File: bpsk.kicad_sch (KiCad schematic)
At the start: 0 parts

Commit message: update bpsk sch
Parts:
- added C1, C8: 47n, symbol Device:C
- added C18: 100n, symbol Device:C
- added C2: 10n, symbol Device:C
- added J1: Screw_Terminal_01x03, symbol Connector:Screw_Terminal_01x03
- added L1: L_Coupled_1243, symbol Device:L_Coupled_1243
- added L2, L3: L_Ferrite, symbol Device:L_Ferrite
- added Q1, Q3, Q6, Q7, Q8, Q9: AO3400A, Package_TO_SOT_SMD:SOT-23, symbol Transistor_FET:AO3400A
- added Q4, Q5: AO3401A, Package_TO_SOT_SMD:SOT-23, symbol Transistor_FET:AO3401A
- added R1, R2: R, symbol Device:R
- added R24, R25, R29, R30: 100, symbol Device:R
- added R26, R3: 3.6k, symbol Device:R
- added R27, R28, R41: 1k, symbol Device:R
- added R31, R32, R36, R38, R46, R47: 47k, symbol Device:R
- added R33, R34, R35, R37, R44, R45: 47, symbol Device:R
- added R39, R48: 68, symbol Device:R
- added R40, R49: 200, symbol Device:R
- added R42, R43: 30k, symbol Device:R
- added R50, R51, R52, R53: 11k, symbol Device:R
- added U1: LM393, symbol Comparator:LM393
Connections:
- new net: Q7.3 (D), R39.1
- new net: C8.2, L1.2
- new net: L1.3, R24.1, R3.1
- new net: L1.4, R25.1, R3.2
- new net: Q9.1 (G), R45.2, R47.1
- new net: Q6.1 (G), R35.2, R36.1
- new net: Q9.3 (D), R49.1
- new net: Q8.1 (G), R44.2, R46.1
- new net: Q3.1 (G), R32.1, R33.2
- new net: Q7.1 (G), R37.2, R38.1
- new net: Q3.3 (D), R29.1
- new net: Q1.1 (G), R31.1, R34.2
- new net: Q1.3 (D), R30.1
- new net: Q4.1 (G), R27.2, R30.2
- new net: Q6.3 (D), R40.1
- new net: Q5.1 (G), R28.2, R29.2
- new net: Q8.3 (D), R48.1
- new net +5V: C18.1, Q4.3 (D), Q5.3 (D), R27.1, R28.1, R42.1, R50.1, R53.1, U1.8 (V+)
- new net FG: J1.3 (Pin_3)
- new net GND: C18.2, C2.2, L1.1, Q1.2 (S), Q3.2 (S), Q6.2 (S), Q7.2 (S), Q8.2 (S), Q9.2 (S), R31.2, R32.2, R36.2, R38.2, R43.2, R46.2, R47.2, R51.2, R52.2, U1.4 (V-)
- new net LC: L2.1, L3.2, R1.2, R2.1, R39.2, R40.2, R48.2, R49.2
- new net LD: L2.2, Q5.2 (S), R2.2
- new net LU: L3.1, Q4.2 (S), R1.1
- new net RX_LEV_H: R44.1
- new net RX_LEV_L: R45.1
- new net RX_SIG: C2.1, C8.1, R42.2, R43.1, R50.2, R51.1, R52.1, R53.2, U1.2 (-), U1.3 (+), U1.5 (+), U1.6 (-)
- new net RX_SIG_H: U1.1
- new net RX_SIG_L: U1.7
- new net S+: C1.1, J1.1 (Pin_1), R24.2, R26.2
- new net S-: C1.2, J1.2 (Pin_2), R25.2, R26.1
- new net TX_FET_D: R33.1
- new net TX_FET_U: R34.1
- new net TX_LEV_H: R37.1
- new net TX_LEV_L: R35.1
- no-connect marks 0 -> 1

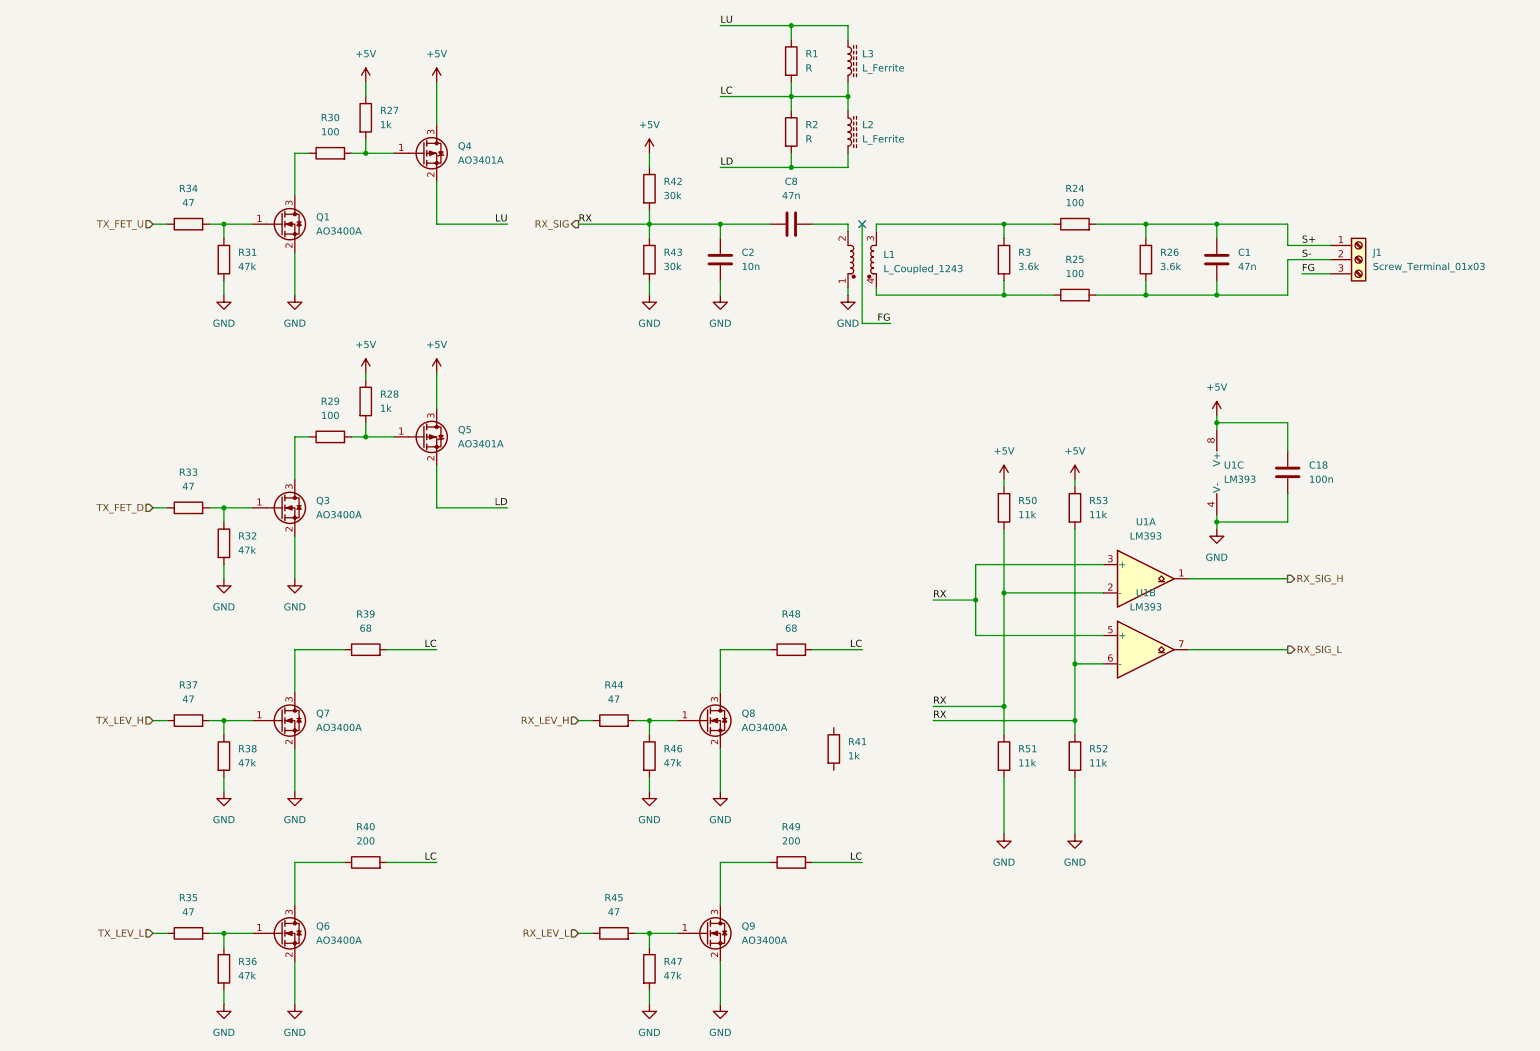
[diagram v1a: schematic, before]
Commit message: add signals
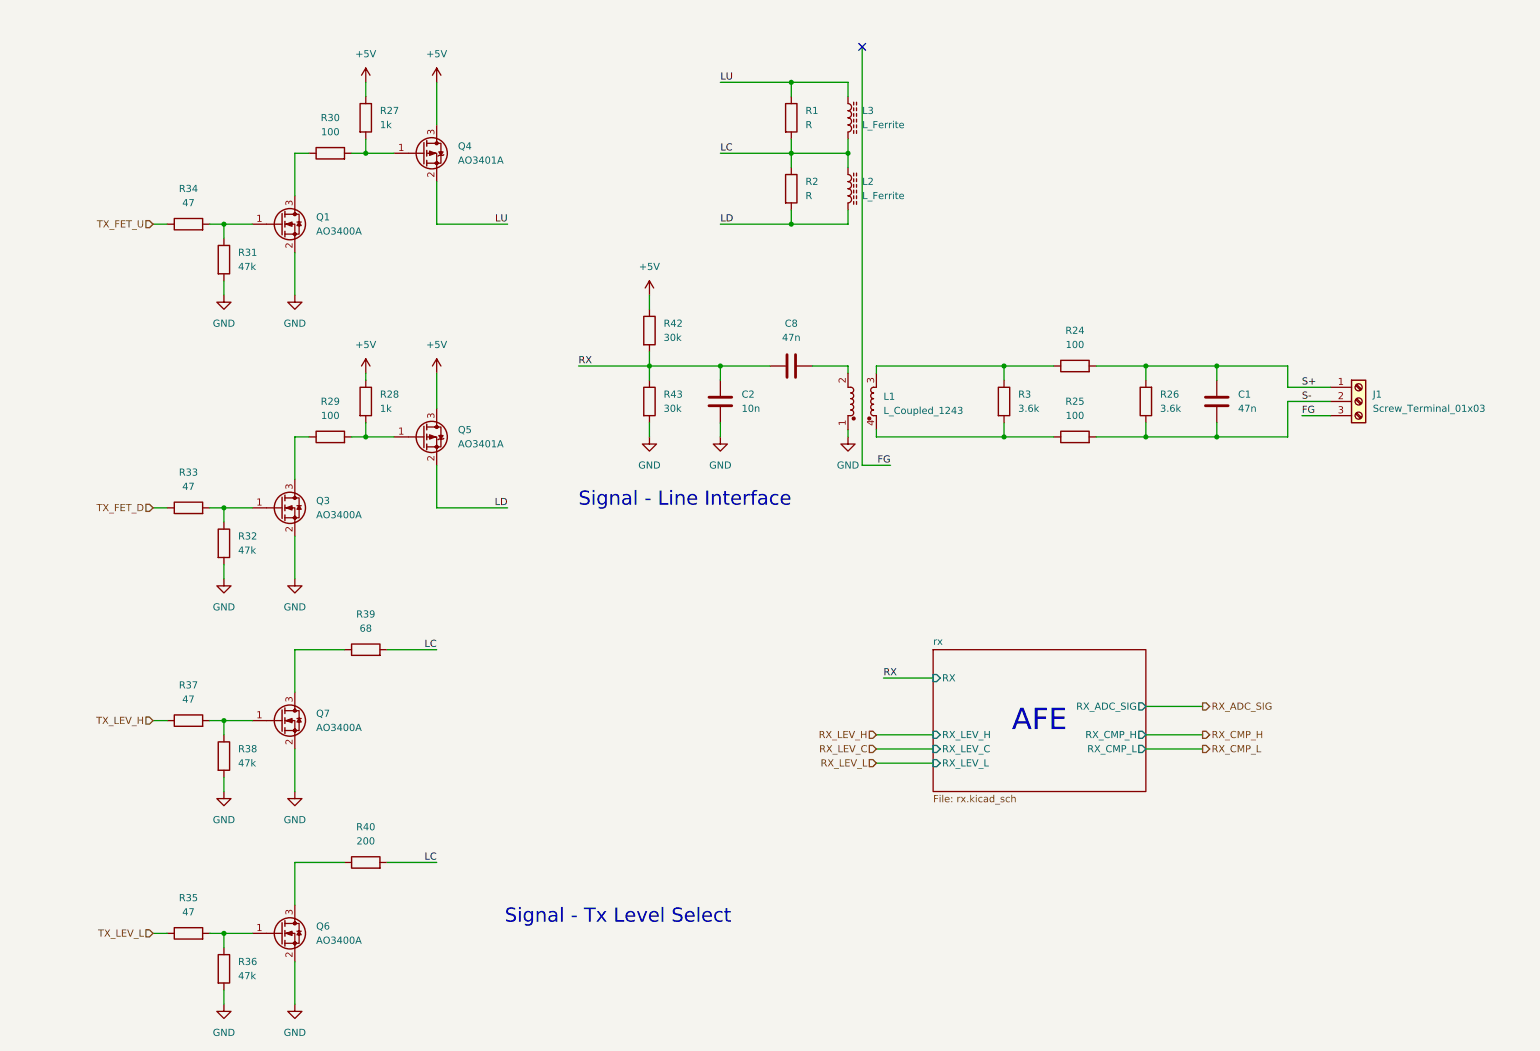
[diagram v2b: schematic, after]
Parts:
- removed C18: 100n, symbol Device:C
- removed Q8, Q9: AO3400A, Package_TO_SOT_SMD:SOT-23, symbol Transistor_FET:AO3400A
- removed R41: 1k, symbol Device:R
- removed R44, R45: 47, symbol Device:R
- removed R46, R47: 47k, symbol Device:R
- removed R48: 68, symbol Device:R
- removed R49: 200, symbol Device:R
- removed R50, R51, R52, R53: 11k, symbol Device:R
- removed U1: LM393, symbol Comparator:LM393
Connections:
- net RX_SIG renamed RX
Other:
- added sheet rx (rx.kicad_sch)
- note added: "AFE"
- note added: "Signal - Line Interface"
- note added: "Signal - Tx Level Select"
- moved on the sheet: C1, C2, C8, J1, L1, L2, L3, R1, R2, R24, R25, R26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

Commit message: update comment
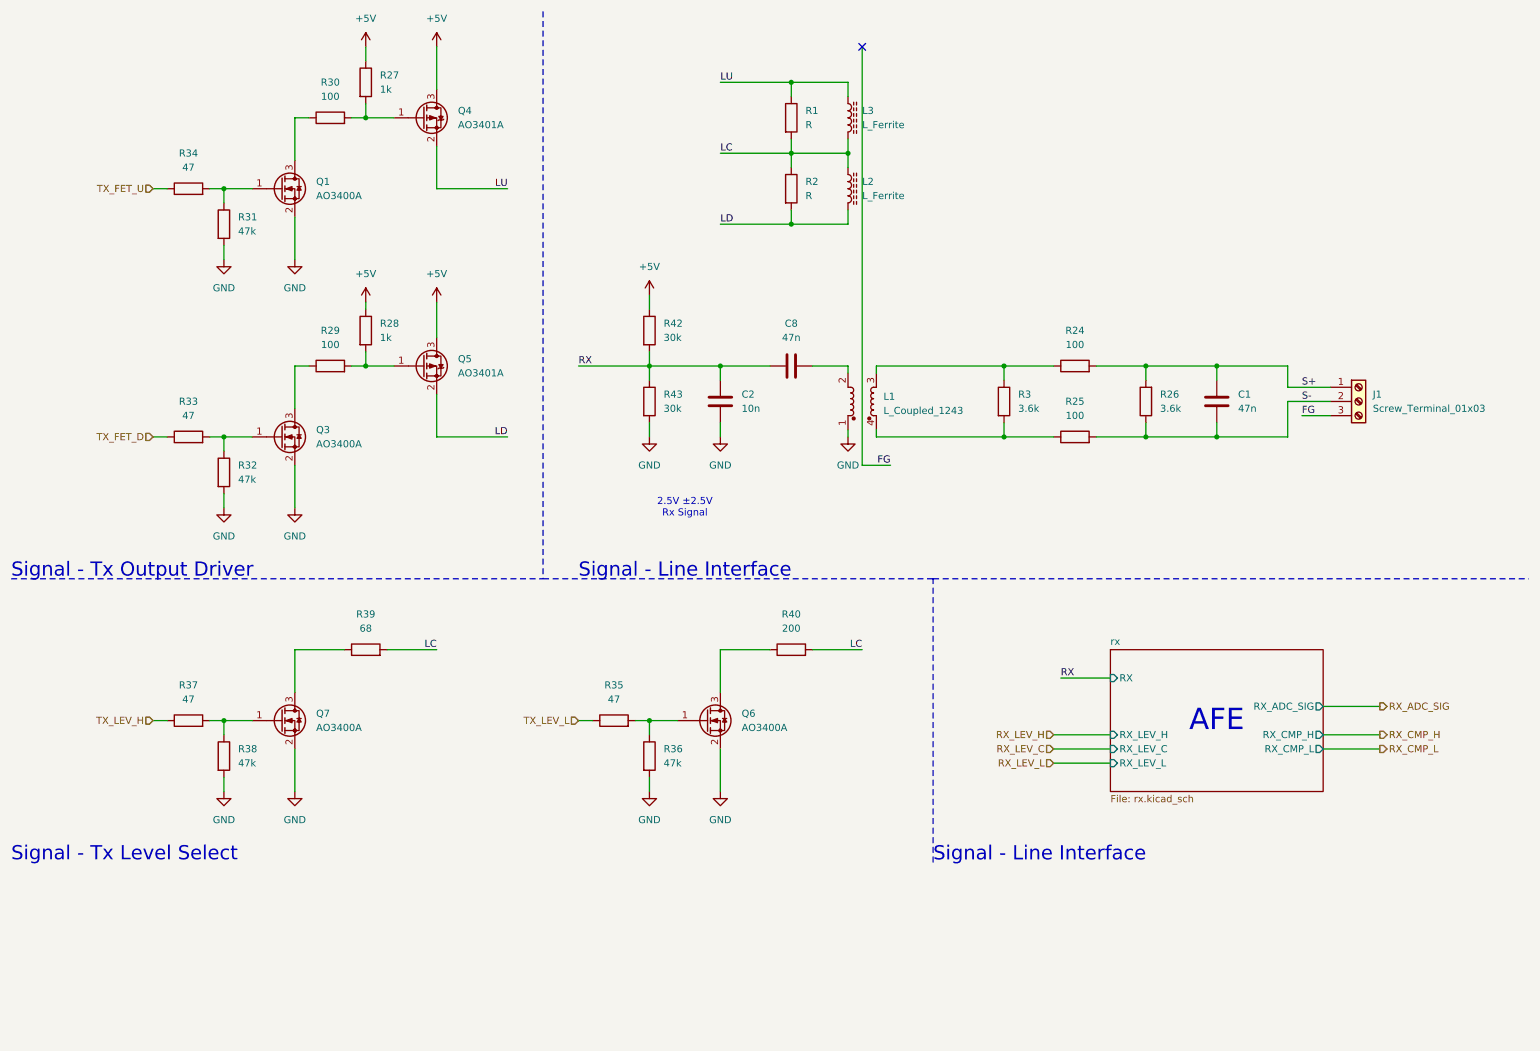
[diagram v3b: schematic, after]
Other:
- note added: "2.5V ±2.5V Rx Signal"
- note added: "Signal - Tx Output Driver"
- moved on the sheet: Q1, Q3, Q4, Q5, Q6, R27, R28, R29, R30, R31, R32, R33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
